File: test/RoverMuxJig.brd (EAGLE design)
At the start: 35.6 x 26.8 mm, 22 parts, among them J1 ISP, Q1 16MHz, U1 ATMEGA328P_TQFP

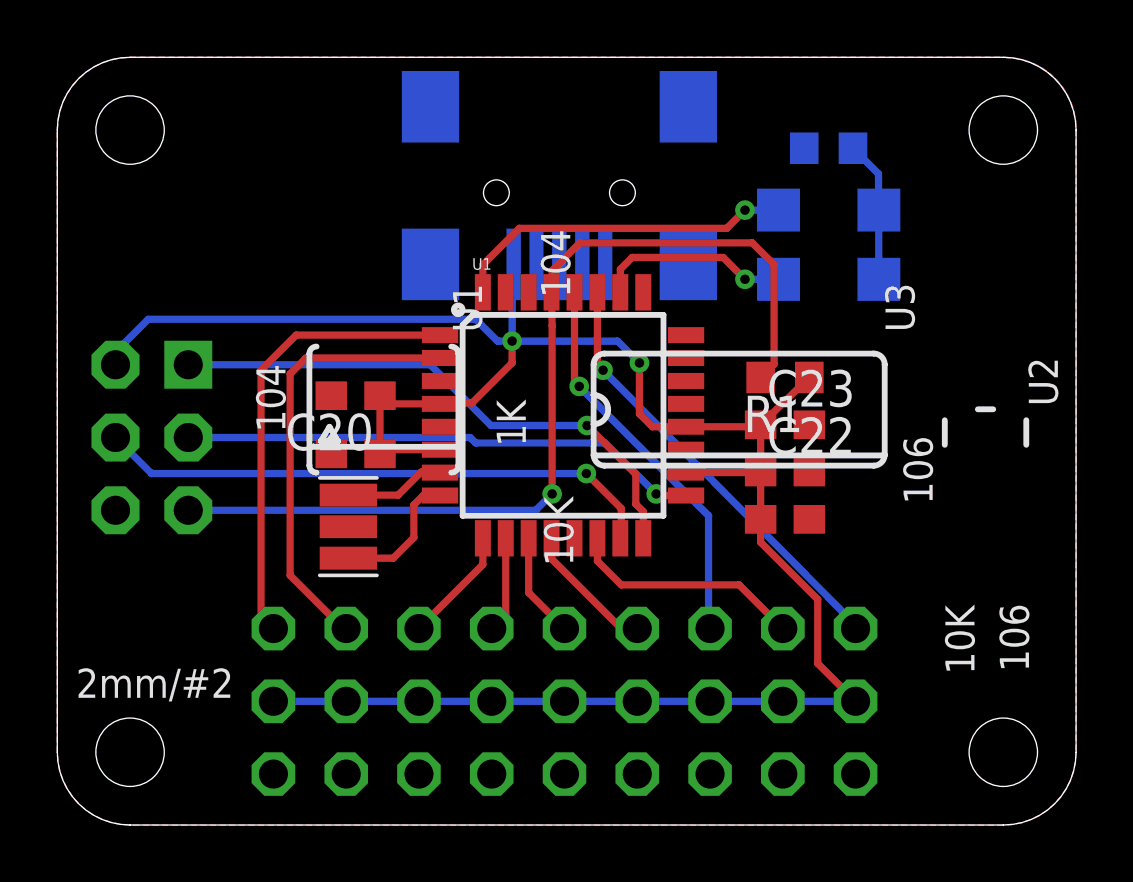
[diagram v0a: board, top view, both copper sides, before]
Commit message: Updated jig
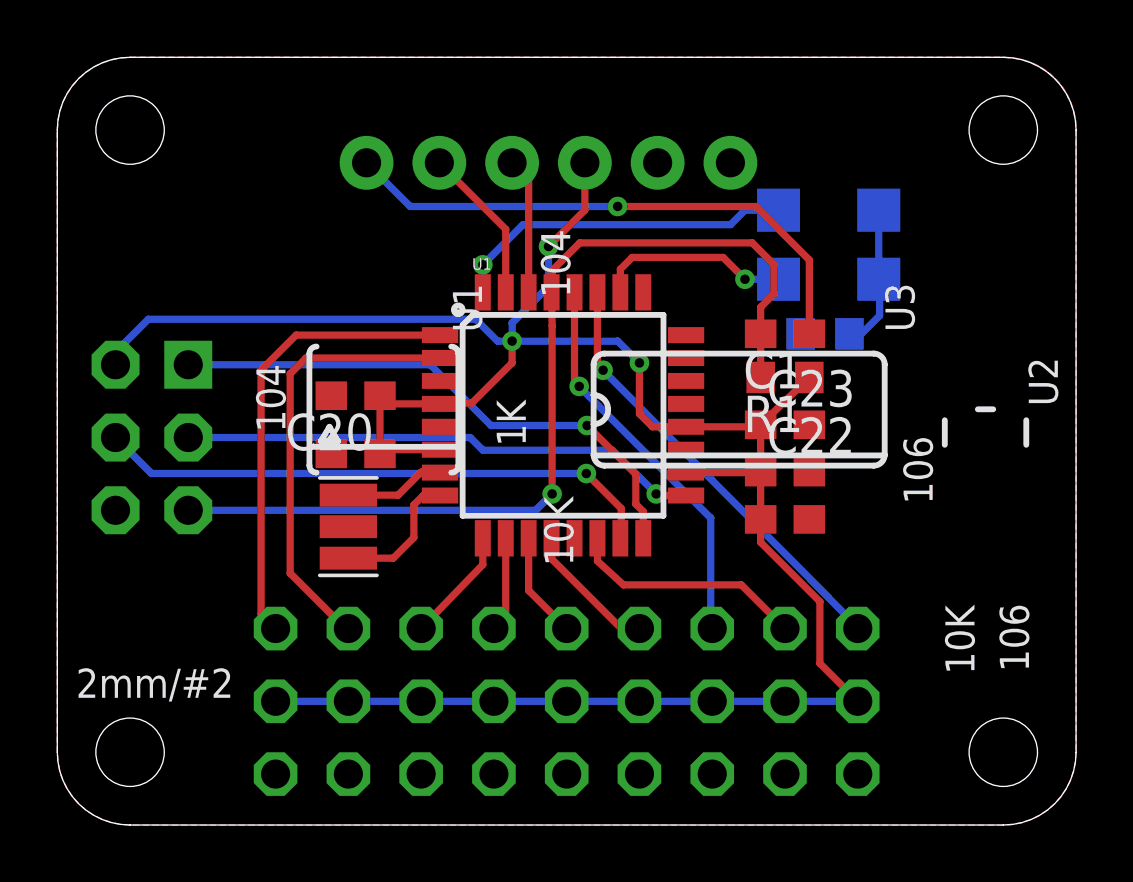
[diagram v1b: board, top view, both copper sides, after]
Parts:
- removed U$4: USB-MINIB-5PIN, SparkFun-Connectors:USB-MINIB
- added C1: 104, rcl:C0603
- added JP1: FTDI, SparkFun-Connectors:FTDI_BASIC
- moved R2 6.48 mm to (26.8, 17.1)
- moved JP11 0.08 mm to (7.62, 4.32)
- moved JP12 0.08 mm to (15.2, 4.32)
- moved JP13 0.08 mm to (22.9, 4.32)
- moved JP21 0.08 mm to (10.2, 4.32)
- moved JP22 0.08 mm to (17.8, 4.32)
- moved JP23 0.08 mm to (25.4, 4.32)
- moved JP31 0.08 mm to (12.7, 4.32)
- moved JP32 0.08 mm to (20.3, 4.32)
- moved JP33 0.08 mm to (27.9, 4.32)
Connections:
- new net N$4: C1.1, JP1.DTR
- new net RX<: JP1.TXO, U1.30
- new net TX>: JP1.RXI, U1.31
- net !RESET: now also C1.2
- net 5V: now also JP1.VCC; no longer U$4.VBUS
- net GND: now also JP1.GND; no longer U$4.GND
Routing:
- net N$4: track 0.00 -> 19.4 mm, vias 0 -> 1
- net TX>: track 0.00 -> 5.48 mm
- net RX<: track 0.00 -> 4.76 mm
- net 5V: track 75.4 -> 80.0 mm, vias 2 -> 3
